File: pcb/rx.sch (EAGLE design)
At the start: 34 parts, among them IC2 STM32F042K6, J1 USB_A_PTH_MALE, Y1 CRYSTAL-26MHZSMD-3.2X2.5

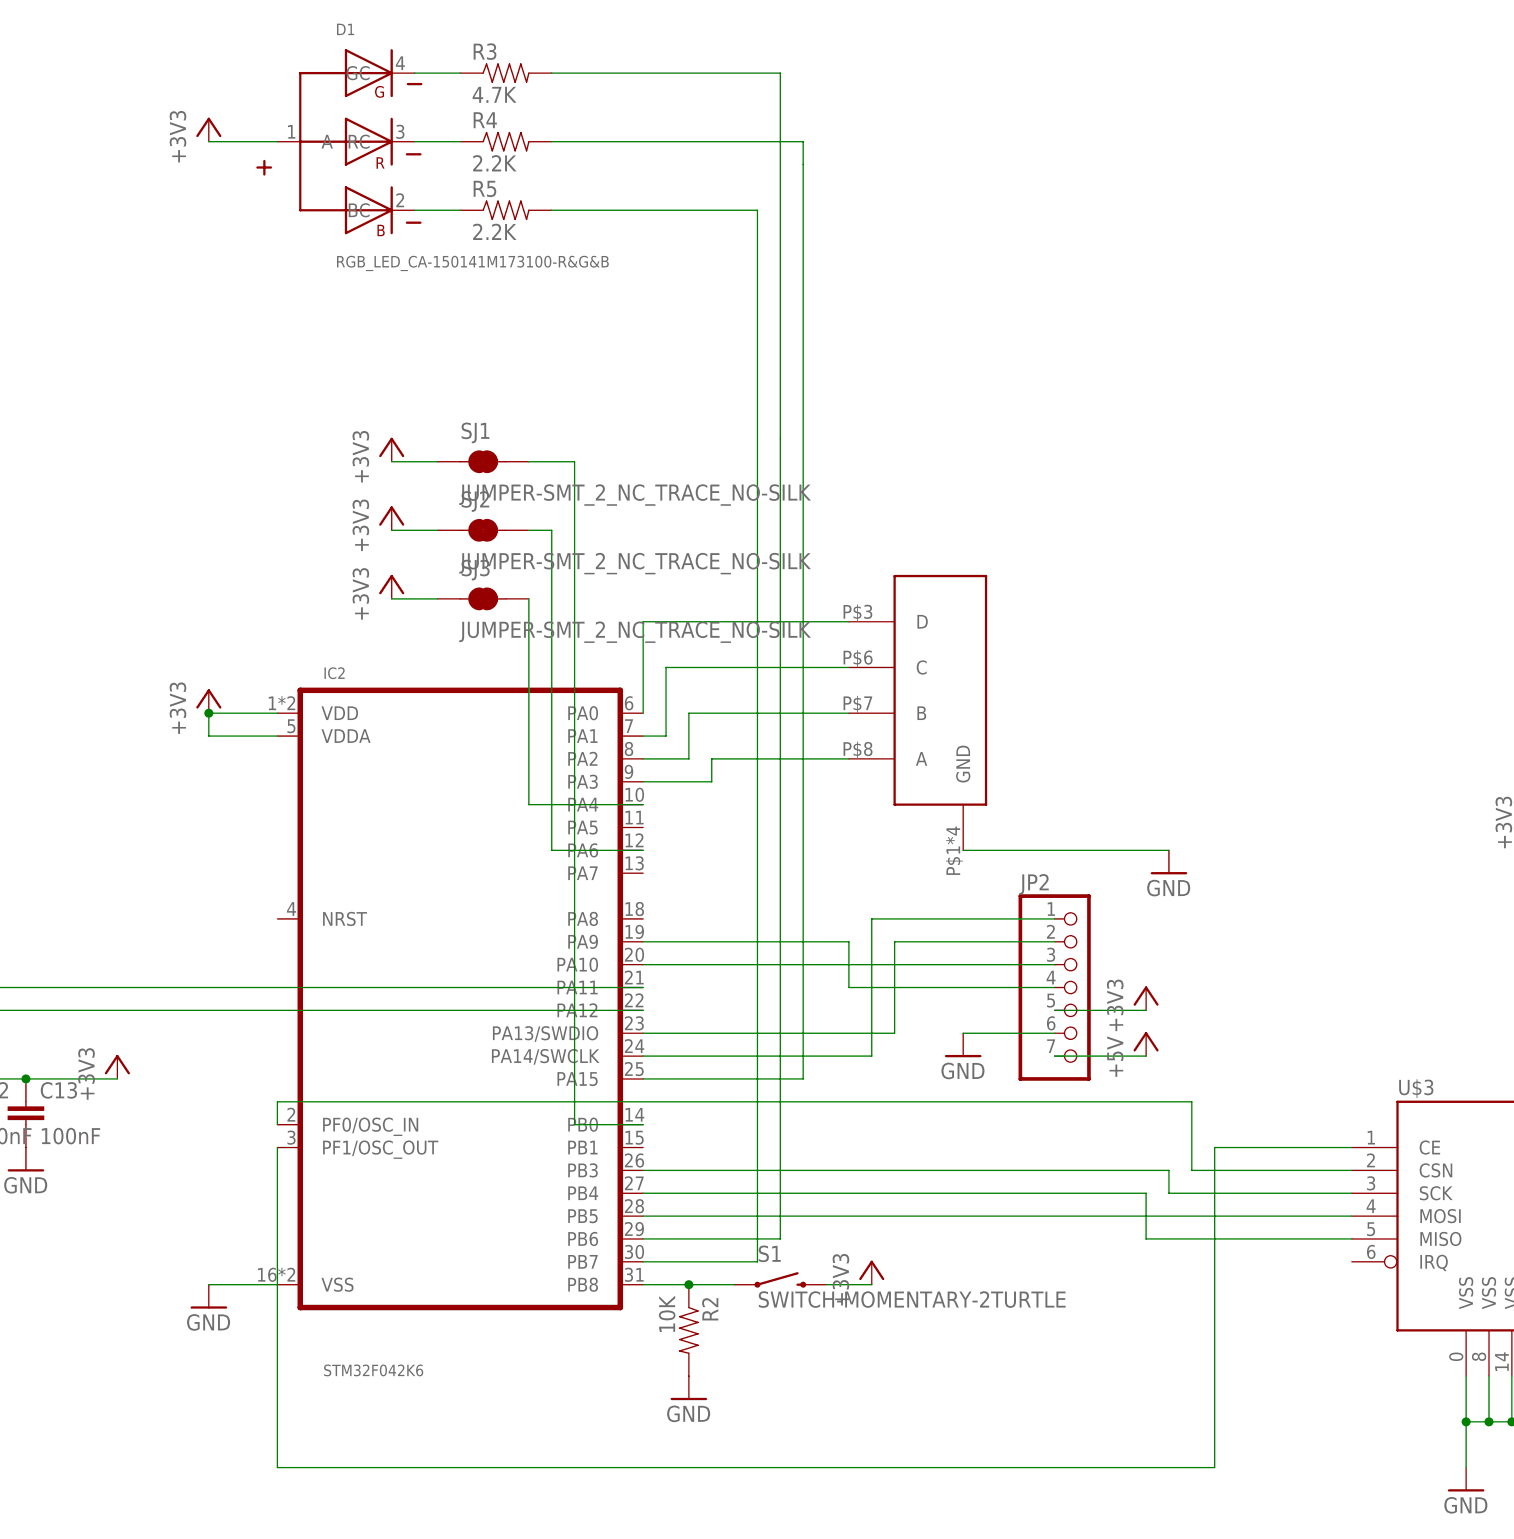
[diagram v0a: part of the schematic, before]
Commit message: further cleanup
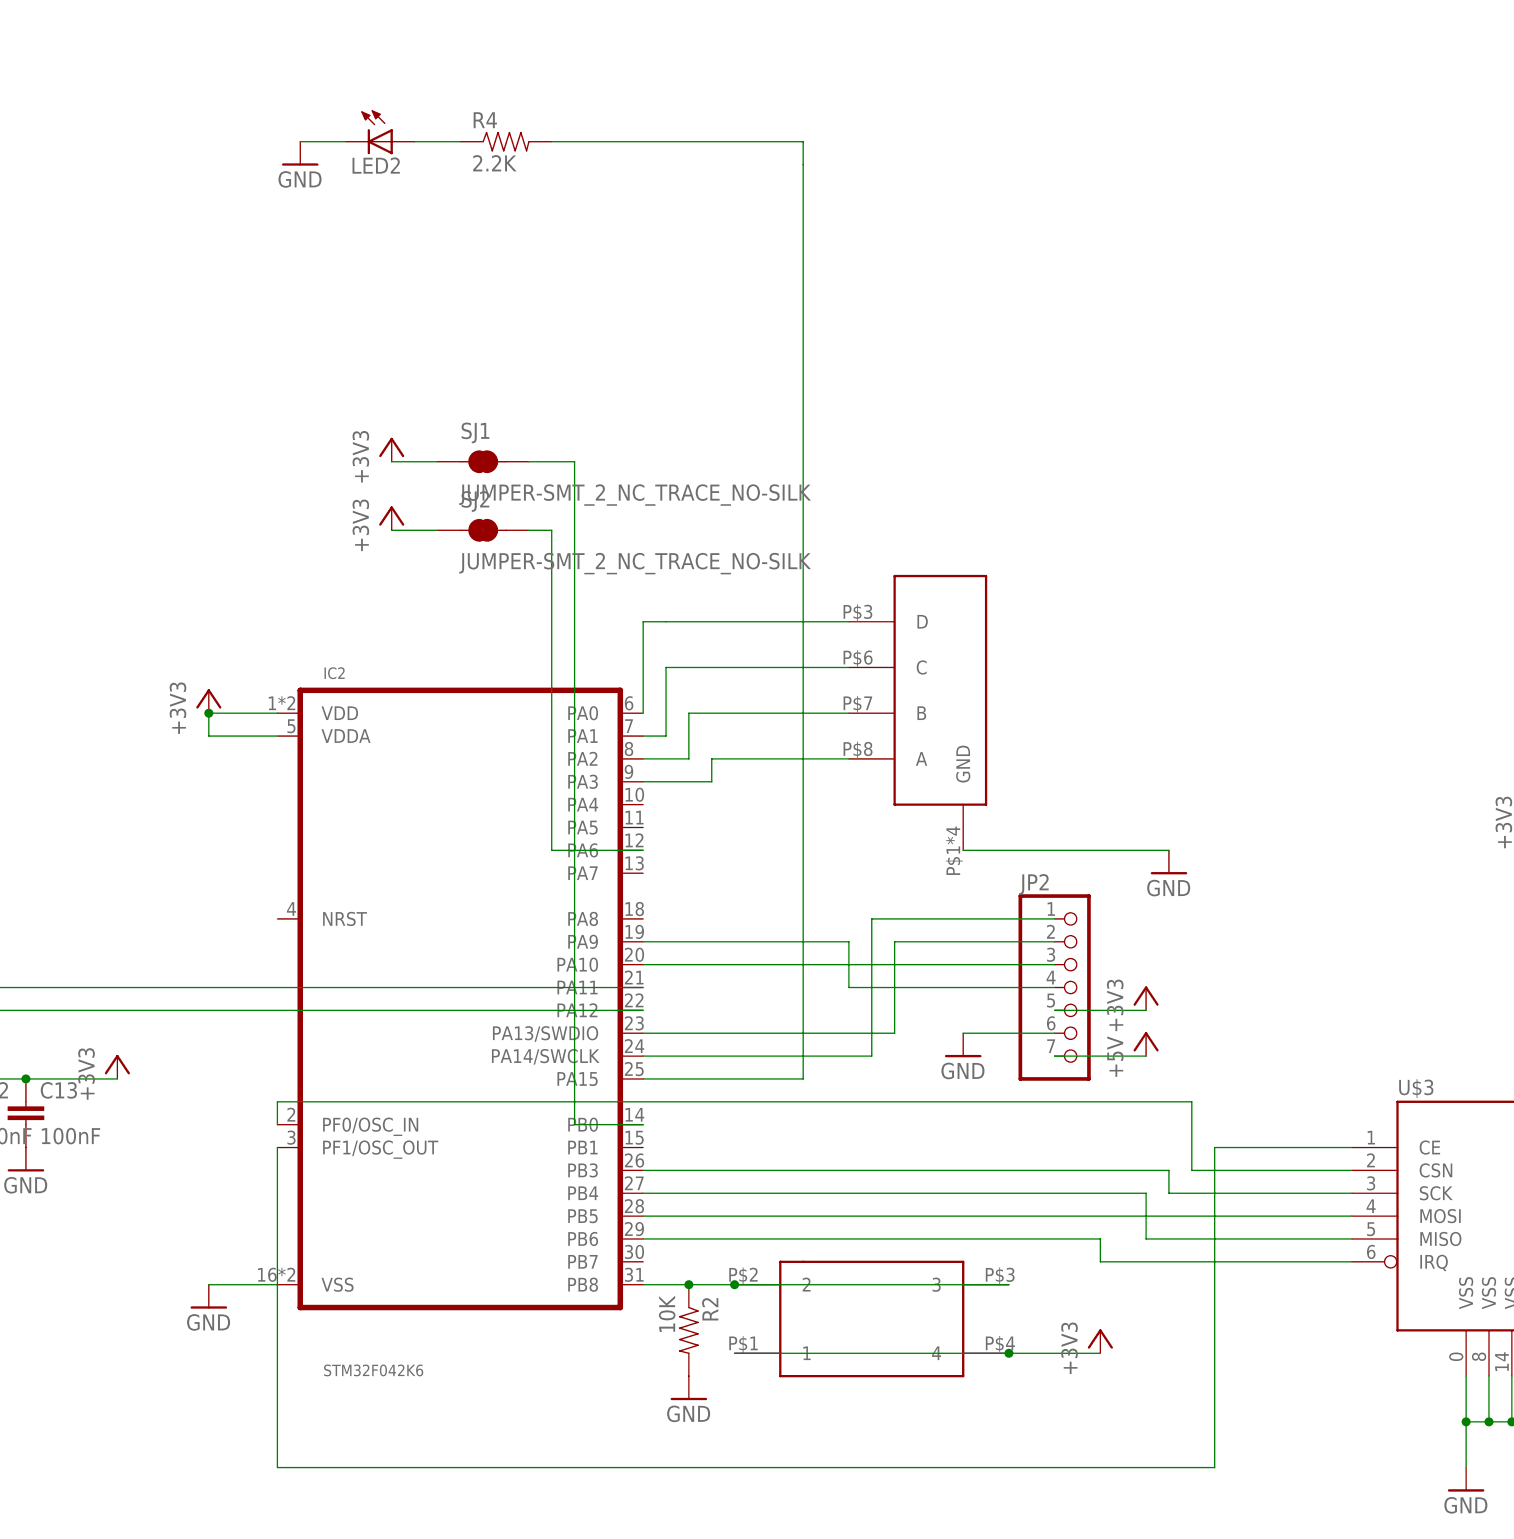
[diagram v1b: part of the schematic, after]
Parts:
- removed D1: RGB_LED_CA-150141M173100-R&G&B, nixx:RGB_LED_CA-150141M173100-R&G&B
- removed R3: 4.7K, joyAnalog:RESISTOR0805-RES
- removed R5: 2.2K, joyAnalog:RESISTOR0805-RES
- removed S1: SWITCH-MOMENTARY-2TURTLE, Adafruit Feather M0 Adalogger:SWITCH-MOMENTARY-2TURTLE
- removed SJ3: JUMPER-SMT_2_NC_TRACE_NO-SILK, SparkFun-Jumpers:JUMPER-SMT_2_NC_TRACE_NO-SILK
- added LED2: (no value), joyAnalog:LEDCHIP-LED0805
- added U$10: 324_SW, 3pos_slide_switch:324_SW
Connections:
- removed net N$19: D1.BC, R5.1
- removed net N$30: IC2.PB6, R3.2
- removed net N$31: IC2.PB7, R5.2
- removed net N$32: IC2.PA4, SJ3.2
- net +3V3: now also U$10.1, U$10.4; no longer D1.A, S1.2, SJ3.1
- net GND: now also LED2.C
- net N$11: now also U$10.2, U$10.3; no longer S1.1
- net N$17: now also IC2.PB6, U$3.IRQ; no longer D1.GC, R3.1
- net N$18: now also LED2.A; no longer D1.RC
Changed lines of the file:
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@@
 <part name="E1" library="SparkFun-RF" deviceset="ANTENNA-GROUNDED" device="TRACE-15.2MM"/>
 <part name="U$1" library="3pos_slide_switch" deviceset="SW_3POS_DEV" device="SW_3POS_OFFICIAL"/>
-<part name="S1" library="Adafruit Feather M0 Adalogger" deviceset="SWITCH-MOMENTARY-2" device="TURTLE"/>
-<part name="D1" library="nixx" deviceset="RGB_LED_CA" device="-150141M173100-R&amp;G&amp;B"/>
 <part name="GND7" library="supply1" library_urn="urn:adsk.eagle:library:371" deviceset="GND" device=""/>
 <part name="+3V1" library="supply1" library_urn="urn:adsk.eagle:library:371" deviceset="+3V3" device=""/>
@@
 <part name="GND19" library="supply1" library_urn="urn:adsk.eagle:library:371" deviceset="GND" device=""/>
 <part name="GND20" library="supply1" library_urn="urn:adsk.eagle:library:371" deviceset="GND" device=""/>
-<part name="R3" library="joyAnalog" deviceset="RESISTOR" device="0805-RES" value="4.7K"/>
 <part name="R4" library="joyAnalog" deviceset="RESISTOR" device="0805-RES" value="2.2K"/>
-<part name="R5" library="joyAnalog" deviceset="RESISTOR" device="0805-RES" value="2.2K"/>
-<part name="+3V4" library="supply1" library_urn="urn:adsk.eagle:library:371" deviceset="+3V3" device=""/>
 <part name="JP2" library="adafruit_changed" deviceset="PINHD-1X8" device="CLEANBIG"/>
 <part name="+3V5" library="supply1" library_urn="urn:adsk.eagle:library:371" deviceset="+3V3" device=""/>
@@
 <part name="SJ1" library="SparkFun-Jumpers" deviceset="JUMPER-SMT_2_NC_TRACE" device="_NO-SILK"/>
 <part name="SJ2" library="SparkFun-Jumpers" deviceset="JUMPER-SMT_2_NC_TRACE" device="_NO-SILK"/>
-<part name="SJ3" library="SparkFun-Jumpers" deviceset="JUMPER-SMT_2_NC_TRACE" device="_NO-SILK"/>
 <part name="+3V6" library="supply1" library_urn="urn:adsk.eagle:library:371" deviceset="+3V3" device=""/>
 <part name="+3V7" library="supply1" library_urn="urn:adsk.eagle:library:371" deviceset="+3V3" device=""/>
-<part name="+3V8" library="supply1" library_urn="urn:adsk.eagle:library:371" deviceset="+3V3" device=""/>
+<part name="U$10" library="3pos_slide_switch" deviceset="324_SW" device=""/>
+<part name="LED2" library="joyAnalog" deviceset="LED" device="CHIP-LED0805"/>
+<part name="GND22" library="supply1" library_urn="urn:adsk.eagle:library:371" deviceset="GND" device=""/>
 </parts>
 <sheets>
@@
 <instance part="E1" gate="G$1" x="294.64" y="-38.1" rot="R270"/>
 <instance part="U$1" gate="G$1" x="106.68" y="15.24" rot="R90"/>
-<instance part="S1" gate="G$1" x="86.36" y="-50.8"/>
-<instance part="D1" gate="G$1" x="40.64" y="76.2"/>
 <instance part="GND7" gate="1" x="-30.48" y="-48.26"/>
 <instance part="+3V1" gate="G$1" x="170.18" y="2.54"/>
@@
 <instance part="R2" gate="G$1" x="76.2" y="-55.88" rot="R270"/>
 <instance part="GND9" gate="1" x="76.2" y="-63.5"/>
-<instance part="+3V2" gate="G$1" x="96.52" y="-48.26"/>
+<instance part="+3V2" gate="G$1" x="121.92" y="-55.88"/>
 <instance part="+3V3" gate="G$1" x="22.86" y="15.24"/>
 <instance part="GND18" gate="1" x="22.86" y="-53.34"/>
@@
 <instance part="GND19" gate="1" x="-5.08" y="-38.1"/>
 <instance part="GND20" gate="1" x="2.54" y="-38.1"/>
-<instance part="R3" gate="G$1" x="55.88" y="83.82"/>
 <instance part="R4" gate="G$1" x="55.88" y="76.2"/>
-<instance part="R5" gate="G$1" x="55.88" y="68.58"/>
-<instance part="+3V4" gate="G$1" x="22.86" y="78.74"/>
 <instance part="JP2" gate="G$1" x="119.38" y="-17.78"/>
 <instance part="+3V5" gate="G$1" x="127" y="-17.78"/>
@@
 <instance part="SJ1" gate="G$1" x="53.34" y="40.64"/>
 <instance part="SJ2" gate="G$1" x="53.34" y="33.02"/>
-<instance part="SJ3" gate="G$1" x="53.34" y="25.4"/>
 <instance part="+3V6" gate="G$1" x="43.18" y="43.18"/>
 <instance part="+3V7" gate="G$1" x="43.18" y="35.56"/>
-<instance part="+3V8" gate="G$1" x="43.18" y="27.94"/>
+<instance part="U$10" gate="G$1" x="96.52" y="-55.88"/>
+<instance part="LED2" gate="G$1" x="43.18" y="76.2" rot="R270"/>
+<instance part="GND22" gate="1" x="33.02" y="73.66"/>
 </instances>
 <busses>
@@
 <wire x1="106.68" y1="-22.86" x2="116.84" y2="-22.86" width="0.1524" layer="91"/>
 </segment>
+<segment>
+<pinref part="GND22" gate="1" pin="GND"/>
+<pinref part="LED2" gate="G$1" pin="C"/>
+<wire x1="33.02" y1="76.2" x2="38.1" y2="76.2" width="0.1524" layer="91"/>
+</segment>
 </net>
 <net name="+3V3" class="0">
@@
 </segment>
 <segment>
-<pinref part="S1" gate="G$1" pin="2"/>
-<pinref part="+3V2" gate="G$1" pin="+3V3"/>
-<wire x1="91.44" y1="-50.8" x2="96.52" y2="-50.8" width="0.1524" layer="91"/>
-</segment>
-<segment>
 <pinref part="+3V3" gate="G$1" pin="+3V3"/>
 <pinref part="IC2" gate="G$1" pin="VDD"/>
@@
 </segment>
 <segment>
-<pinref part="D1" gate="G$1" pin="A"/>
-<pinref part="+3V4" gate="G$1" pin="+3V3"/>
-<wire x1="30.48" y1="76.2" x2="22.86" y2="76.2" width="0.1524" layer="91"/>
-</segment>
-<segment>
 <pinref part="JP2" gate="G$1" pin="5"/>
 <pinref part="+3V5" gate="G$1" pin="+3V3"/>
@@
 </segment>
 <segment>
-<pinref part="+3V8" gate="G$1" pin="+3V3"/>
-<pinref part="SJ3" gate="G$1" pin="1"/>
-<wire x1="43.18" y1="25.4" x2="48.26" y2="25.4" width="0.1524" layer="91"/>
+<pinref part="U$10" gate="G$1" pin="4"/>
+<pinref part="+3V2" gate="G$1" pin="+3V3"/>
+<wire x1="111.76" y1="-58.42" x2="121.92" y2="-58.42" width="0.1524" layer="91"/>
+<pinref part="U$10" gate="G$1" pin="1"/>
+<wire x1="111.76" y1="-58.42" x2="81.28" y2="-58.42" width="0.1524" layer="91"/>
+<junction x="111.76" y="-58.42"/>
 </segment>
 </net>
@@
 <segment>
 <pinref part="IC2" gate="G$1" pin="PB8"/>
-<pinref part="S1" gate="G$1" pin="1"/>
 <wire x1="71.12" y1="-50.8" x2="76.2" y2="-50.8" width="0.1524" layer="91"/>
 <pinref part="R2" gate="G$1" pin="1"/>
+<pinref part="U$10" gate="G$1" pin="2"/>
 <wire x1="76.2" y1="-50.8" x2="81.28" y2="-50.8" width="0.1524" layer="91"/>
 <junction x="76.2" y="-50.8"/>
+<pinref part="U$10" gate="G$1" pin="3"/>
+<wire x1="81.28" y1="-50.8" x2="111.76" y2="-50.8" width="0.1524" layer="91"/>
+<junction x="81.28" y="-50.8"/>
 </segment>
 </net>
@@
 </segment>
 </net>
-<net name="N$17" class="0">
-<segment>
-<pinref part="D1" gate="G$1" pin="GC"/>
-<pinref part="R3" gate="G$1" pin="1"/>
-<wire x1="45.72" y1="83.82" x2="50.8" y2="83.82" width="0.1524" layer="91"/>
-</segment>
-</net>
 <net name="N$18" class="0">
 <segment>
-<pinref part="D1" gate="G$1" pin="RC"/>
 <pinref part="R4" gate="G$1" pin="1"/>
 <wire x1="45.72" y1="76.2" x2="50.8" y2="76.2" width="0.1524" layer="91"/>
-</segment>
-</net>
-<net name="N$19" class="0">
-<segment>
-<pinref part="D1" gate="G$1" pin="BC"/>
-<pinref part="R5" gate="G$1" pin="1"/>
-<wire x1="45.72" y1="68.58" x2="50.8" y2="68.58" width="0.1524" layer="91"/>
+<pinref part="LED2" gate="G$1" pin="A"/>
 </segment>
 </net>
@@
 </segment>
 </net>
-<net name="N$30" class="0">
-<segment>
-<pinref part="IC2" gate="G$1" pin="PB6"/>
-<wire x1="71.12" y1="-45.72" x2="86.36" y2="-45.72" width="0.1524" layer="91"/>
-<wire x1="86.36" y1="-45.72" x2="86.36" y2="43.18" width="0.1524" layer="91"/>
-<pinref part="R3" gate="G$1" pin="2"/>
-<wire x1="86.36" y1="43.18" x2="86.36" y2="83.82" width="0.1524" layer="91"/>
-<wire x1="86.36" y1="83.82" x2="60.96" y2="83.82" width="0.1524" layer="91"/>
-</segment>
-</net>
-<net name="N$31" class="0">
-<segment>
-<pinref part="IC2" gate="G$1" pin="PB7"/>
-<wire x1="71.12" y1="-48.26" x2="83.82" y2="-48.26" width="0.1524" layer="91"/>
-<wire x1="83.82" y1="-48.26" x2="83.82" y2="68.58" width="0.1524" layer="91"/>
-<pinref part="R5" gate="G$1" pin="2"/>
-<wire x1="83.82" y1="68.58" x2="60.96" y2="68.58" width="0.1524" layer="91"/>
-</segment>
-</net>
-<net name="N$32" class="0">
-<segment>
-<pinref part="IC2" gate="G$1" pin="PA4"/>
-<pinref part="SJ3" gate="G$1" pin="2"/>
-<wire x1="71.12" y1="2.54" x2="58.42" y2="2.54" width="0.1524" layer="91"/>
-<wire x1="58.42" y1="2.54" x2="58.42" y2="25.4" width="0.1524" layer="91"/>
-</segment>
-</net>
 <net name="N$33" class="0">
 <segment>
@@
 </segment>
 </net>
+<net name="N$17" class="0">
+<segment>
+<pinref part="IC2" gate="G$1" pin="PB6"/>
+<wire x1="71.12" y1="-45.72" x2="121.92" y2="-45.72" width="0.1524" layer="91"/>
+<wire x1="121.92" y1="-45.72" x2="121.92" y2="-48.26" width="0.1524" layer="91"/>
+<pinref part="U$3" gate="G$1" pin="IRQ"/>
+<wire x1="121.92" y1="-48.26" x2="149.86" y2="-48.26" width="0.1524" layer="91"/>
+</segment>
+</net>
